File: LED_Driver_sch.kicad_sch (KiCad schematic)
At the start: 33 parts, among them J7 12V IN, J8 12V RGB LED, Q1 PMOS, Q2 NMOS, Q3 NMOS, Q4 NMOS, U6 TLV9001TIDCKR

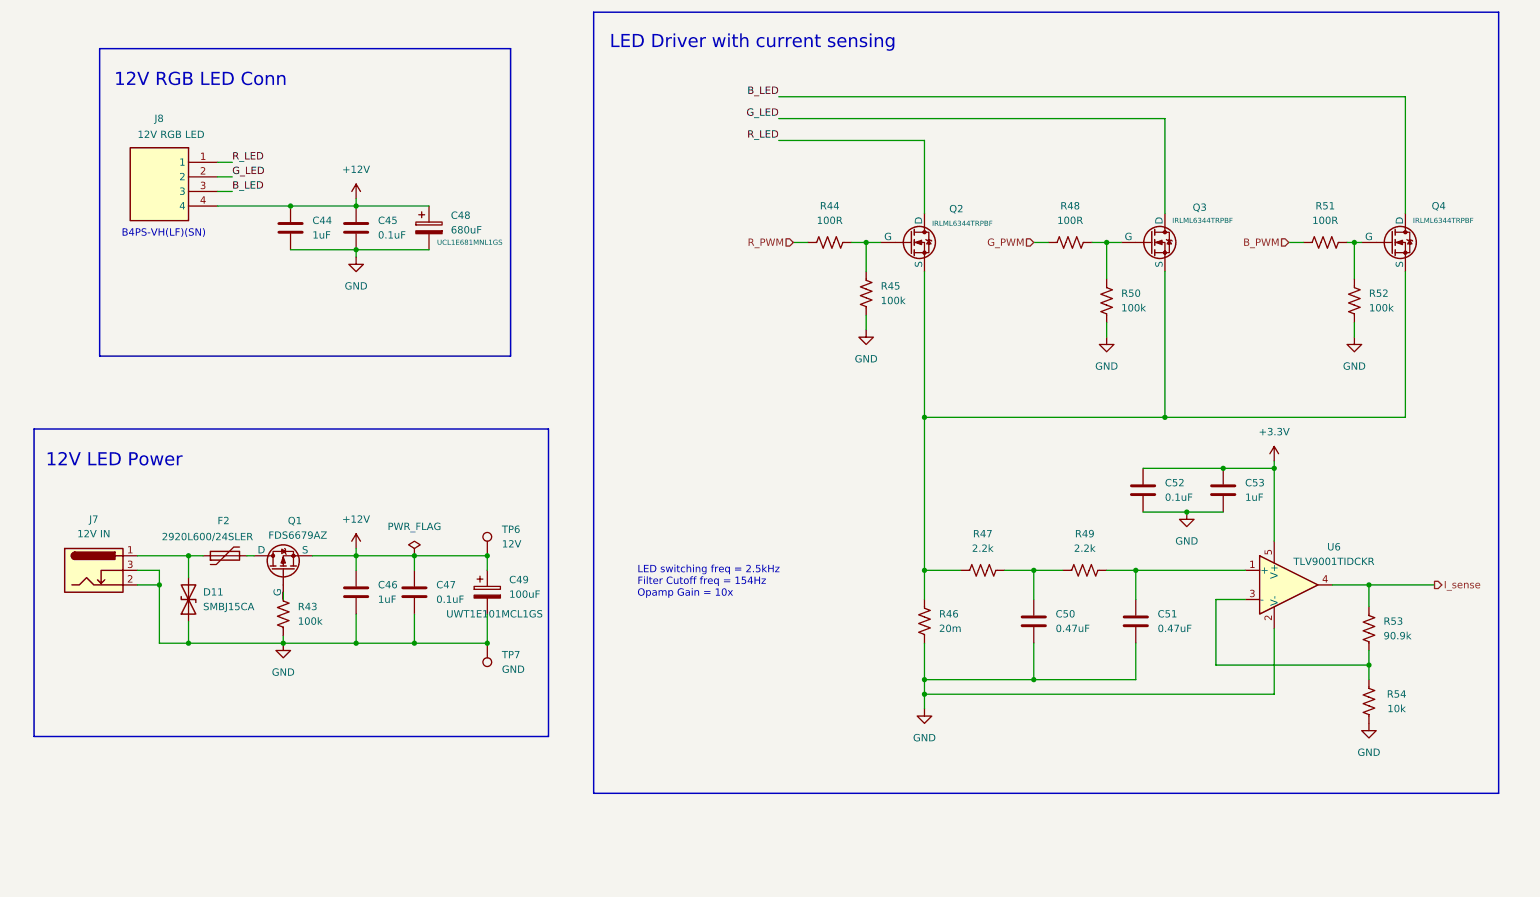
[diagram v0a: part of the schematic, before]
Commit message: Layout Routing
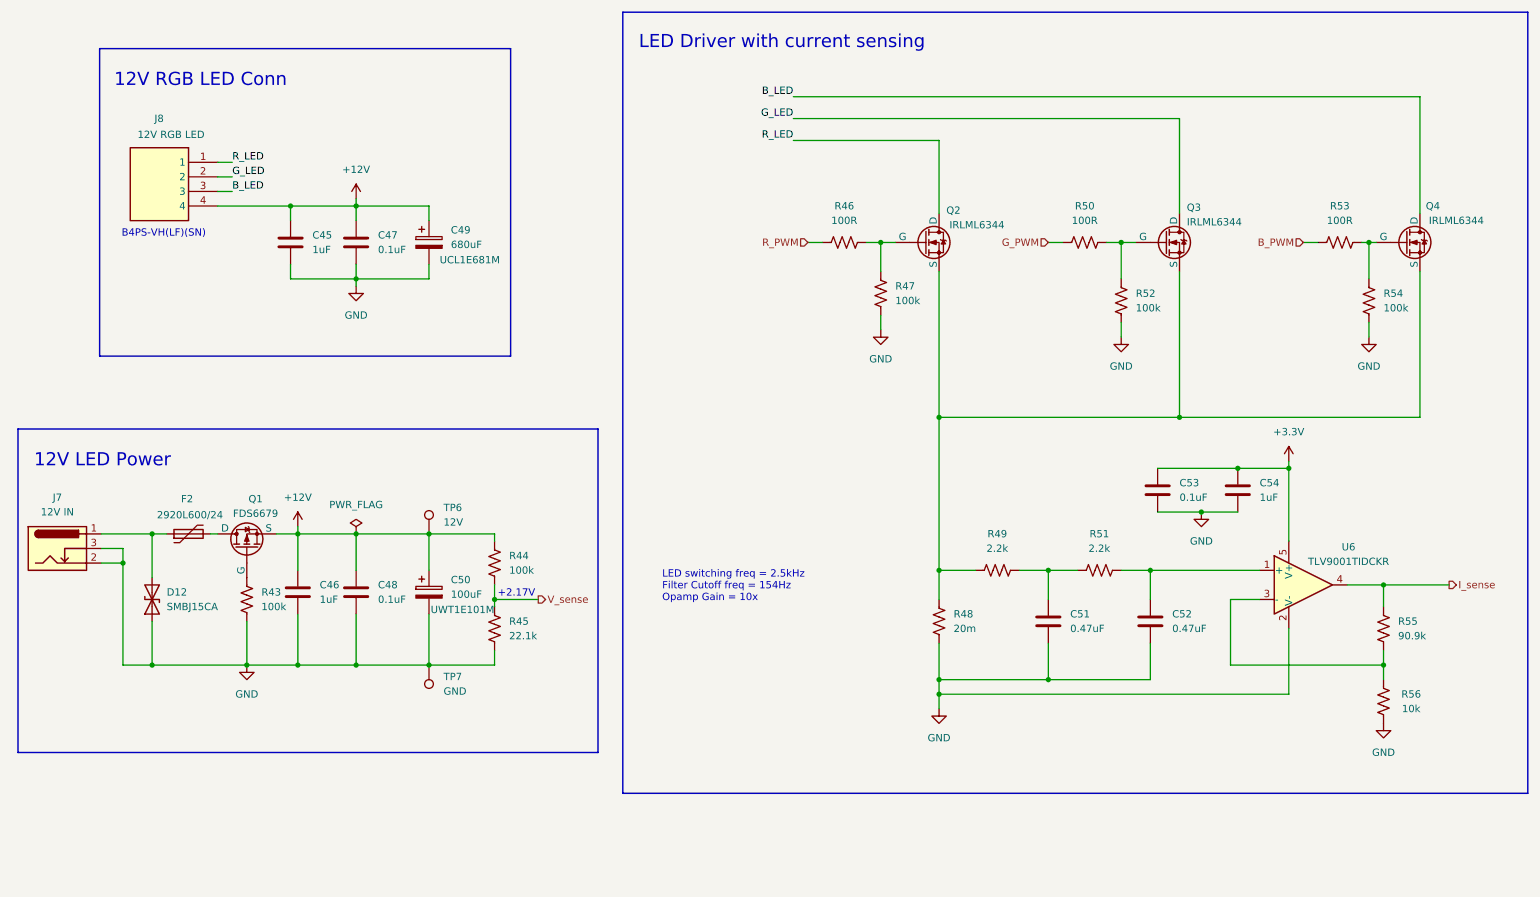
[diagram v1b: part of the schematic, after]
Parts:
- added R44: 100k, Resistor_SMD:R_0603_1608Metric, symbol Device:R_US
- added R45: 22.1k, Resistor_SMD:R_0603_1608Metric, symbol Device:R_US
- C49: renamed from C48; MPN UCL1E681MNL1GS -> UCL1E681M
- C50: renamed from C49; MPN UWT1E101MCL1GS -> UWT1E101M
- F2: MPN 2920L600/24SLER -> 2920L600/24
- Q1: MPN FDS6679AZ -> FDS6679
- Q2, Q3, Q4: MPN IRLML6344TRPBF -> IRLML6344
- renumbered C44 to C45, C45 to C47, C47 to C48, C50 to C51, C51 to C52, C52 to C53, C53 to C54, D11 to D12, R44 to R46, R45 to R47, R46 to R48, R47 to R49, R48 to R50, R49 to R51, R50 to R52, R51 to R53, R52 to R54, R53 to R55, R54 to R56
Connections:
- net +12V: now also R44.1
- net GND: now also R45.2
- new net V_sense: R44.2, R45.1
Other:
- note added: "+2.17V"
- moved on the sheet: C45, C46, C47, C48, C49, C50, C51, C52, C53, C54, D12, F2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
